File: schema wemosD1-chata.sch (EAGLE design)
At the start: 10 parts

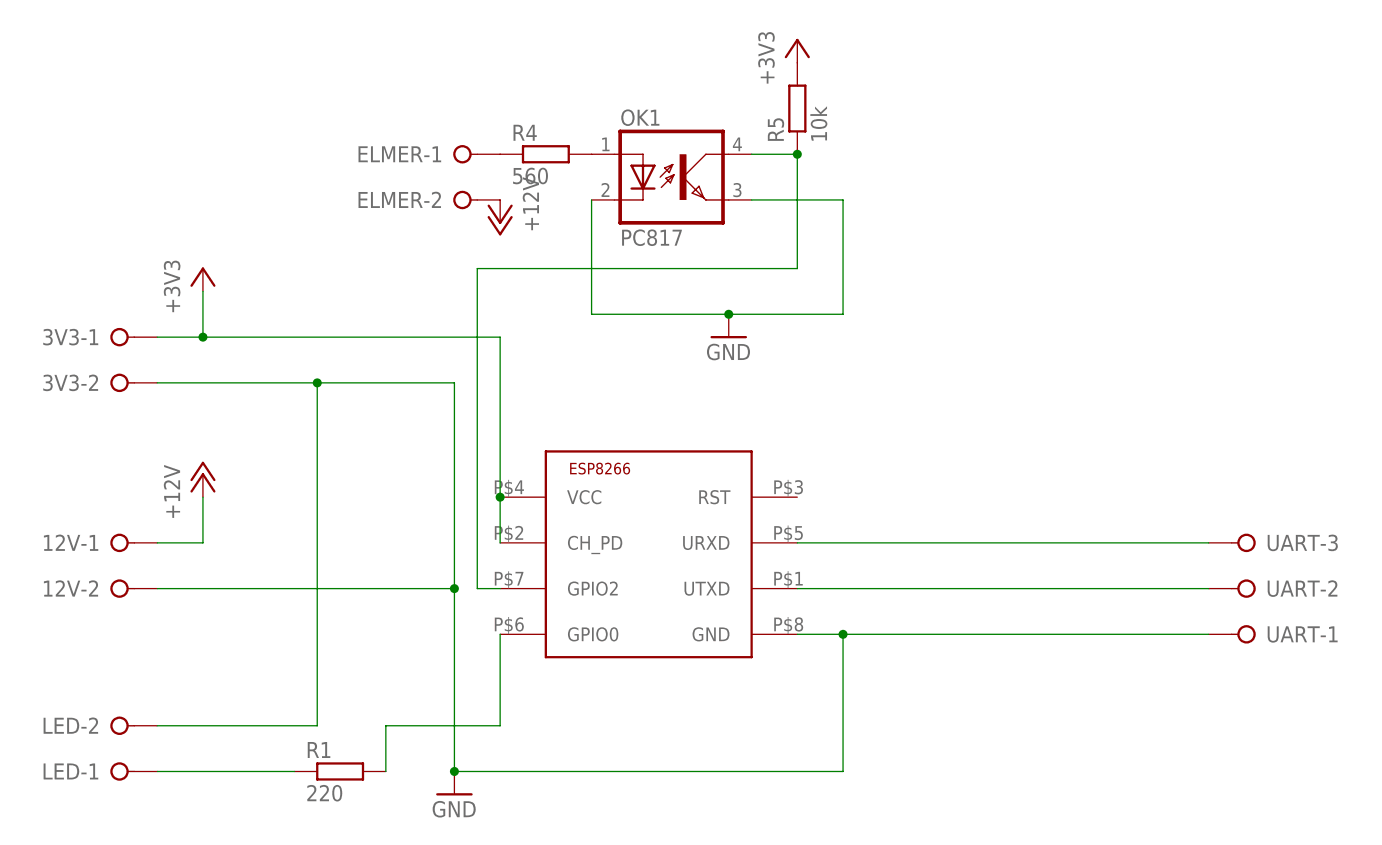
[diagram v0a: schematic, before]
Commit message: +
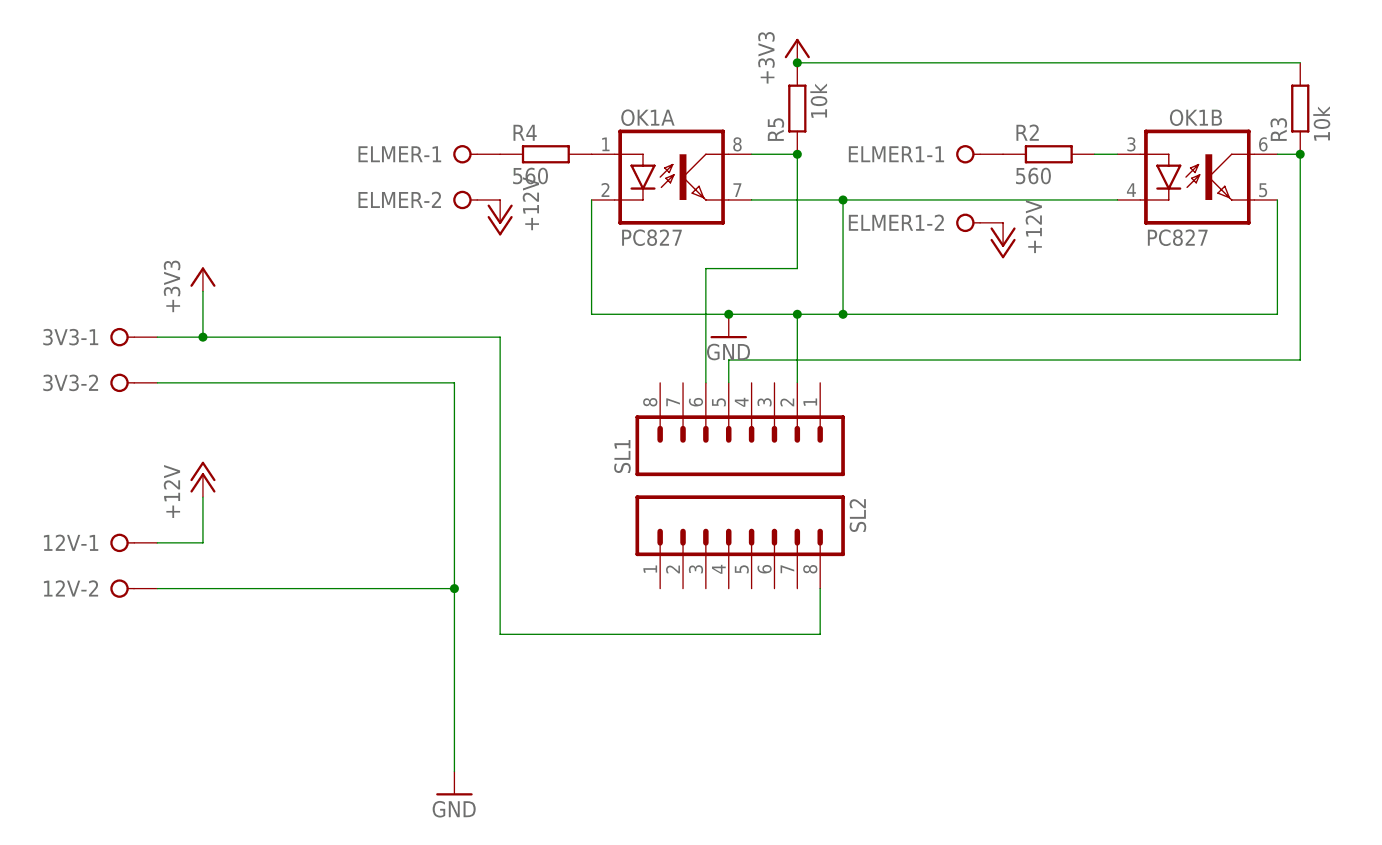
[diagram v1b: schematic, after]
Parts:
- removed LED: (no value), con-wago-508:W237-02P
- removed R1: 220, rcl:R-EU_0204/7
- removed U$1: ESP8266-01, ESP8266:ESP8266-01
- removed UART: (no value), con-wago-508:W237-3E
- added ELMER1: (no value), con-wago-508:W237-02P
- added R2: 560, rcl:R-EU_0204/7
- added R3: 10k, rcl:R-EU_0204/7
- added SL1, SL2: (no value), con-amp-quick:M08
- OK1: value PC817 -> PC827; device optocoupler:PC817 -> optocoupler:PC827
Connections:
- removed net N$3: R1.2, U$1.GPIO0
- removed net N$5: U$1.URXD, UART-3.KL
- removed net N$6: U$1.UTXD, UART-2.KL
- new net N$1: OK1A.A, R4.2
- new net N$9: OK1B.COL, R3.1, SL1.5
- net +12V: now also ELMER1-2.KL
- net +3V3: now also R3.2, SL2.8; no longer U$1.CH_PD, U$1.VCC
- net GND: now also OK1A.C, OK1A.EMIT, OK1B.C, OK1B.EMIT, SL1.2; no longer LED-2.KL, OK1.C, OK1.EMIT, U$1.GND, UART-1.KL
- net N$2: now also ELMER1-1.KL, R2.1; no longer LED-1.KL, R1.1
- net N$4: now also OK1B.A, R2.2; no longer OK1.A, R4.2
- net N$7: now also OK1A.COL, SL1.6; no longer OK1.COL, U$1.GPIO2
